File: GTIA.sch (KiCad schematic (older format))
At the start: 72 parts, among them J2 Video, Q1 2N3904, Q2 2N3904, Q3 2N3904, Q6 2N3904, U17 GTIA, U18 74LS08, U20 4050, U21 74LS74, Y2 4,43 MHz

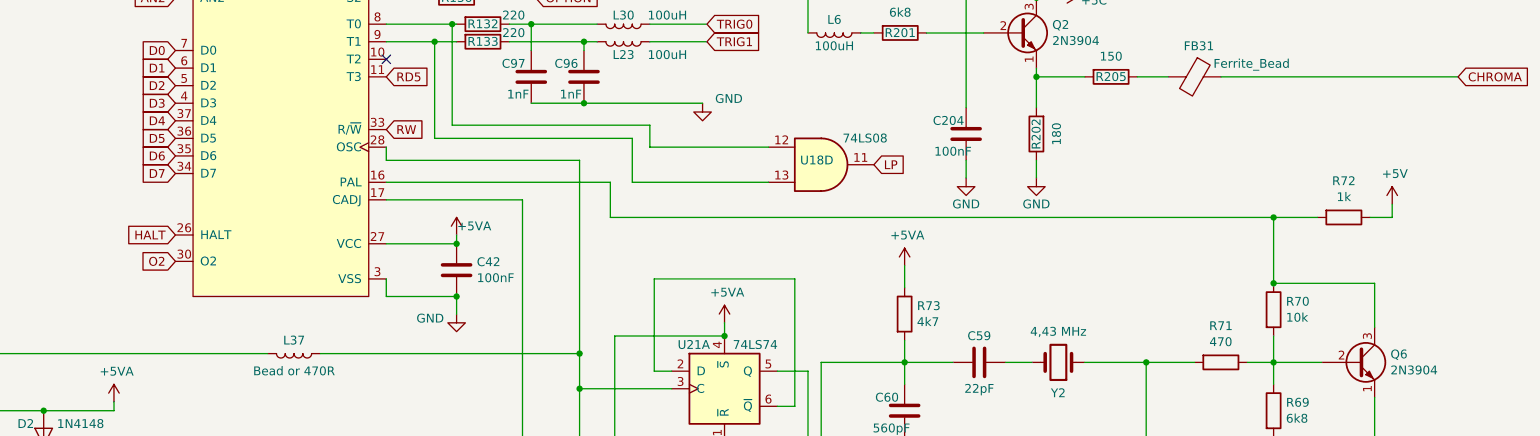
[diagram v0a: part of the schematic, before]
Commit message: Tracking
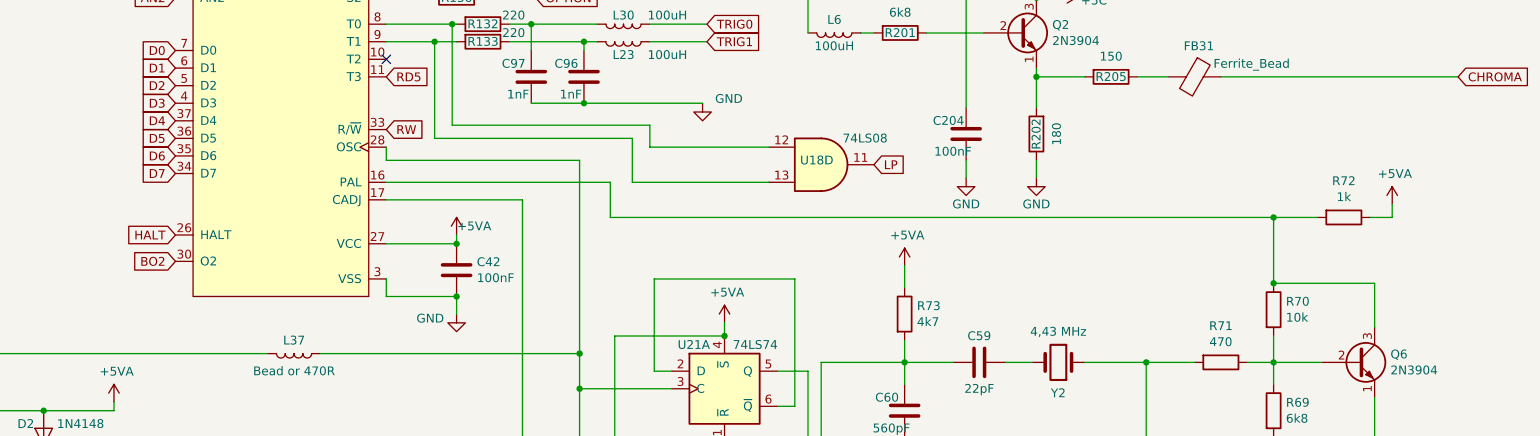
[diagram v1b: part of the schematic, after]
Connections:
- net +5V is gone; now on net +5VA: R72.1
- net O2 renamed BO2
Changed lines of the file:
@@
 HALT
 Text GLabel 3125 4675 0    50   Input ~ 0
-O2
+BO2
 Text GLabel 3125 2075 0    50   Input ~ 0
 GTIA
@@
 MONO
 $Comp
-L power:+5V #PWR0163
-U 1 1 602CA007
-P 10050 4350
-F 0 "#PWR0163" H 10050 4200 50  0001 C CNN
-F 1 "+5V" H 10065 4523 50  0000 C CNN
-F 2 "" H 10050 4350 50  0001 C CNN
-F 3 "" H 10050 4350 50  0001 C CNN
-	1    10050 4350
-	1    0    0    -1
-$EndComp
-$Comp
 L Device:C C204
 U 1 1 60308154
@@
 Wire Wire Line
 	9600 1900 9300 1900
+$Comp
+L power:+5VA #PWR0163
+U 1 1 6036AA54
+P 10050 4350
+F 0 "#PWR0163" H 10050 4200 50  0001 C CNN
+F 1 "+5VA" H 10065 4523 50  0000 C CNN
+F 2 "" H 10050 4350 50  0001 C CNN
+F 3 "" H 10050 4350 50  0001 C CNN
+	1    10050 4350
+	1    0    0    -1
+$EndComp
 $EndSCHEMATC
